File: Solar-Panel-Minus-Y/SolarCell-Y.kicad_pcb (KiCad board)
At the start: 6 copper layers, 64 x 58 mm, 67 parts, among them IC2 TSL2561, J1 XF2M-1015-1A, J3 BATTERY CONNECTOR, J4 B2B-PH-SM4-TB_LF__SN_, U2 Value, U3 SW_SPDT, U4 SW_SPDT

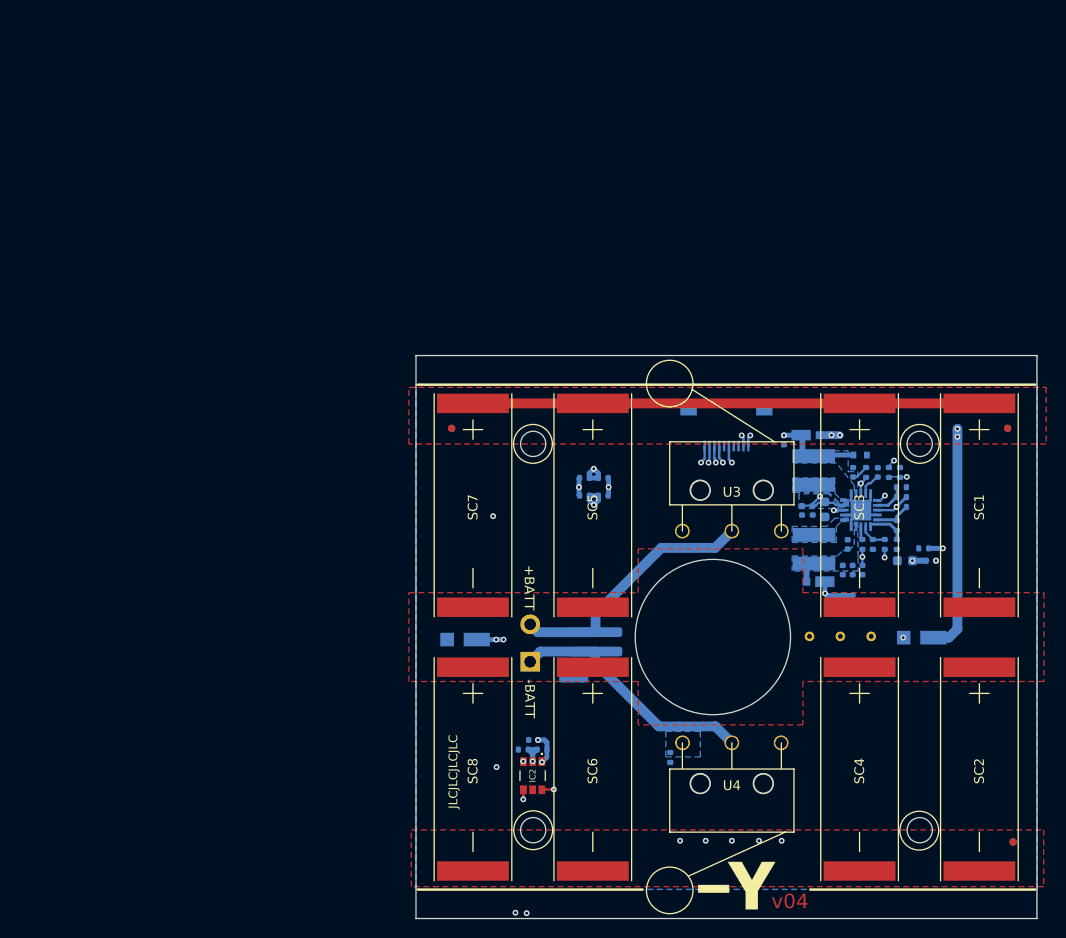
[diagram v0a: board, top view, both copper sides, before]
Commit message: Made Requested Changes
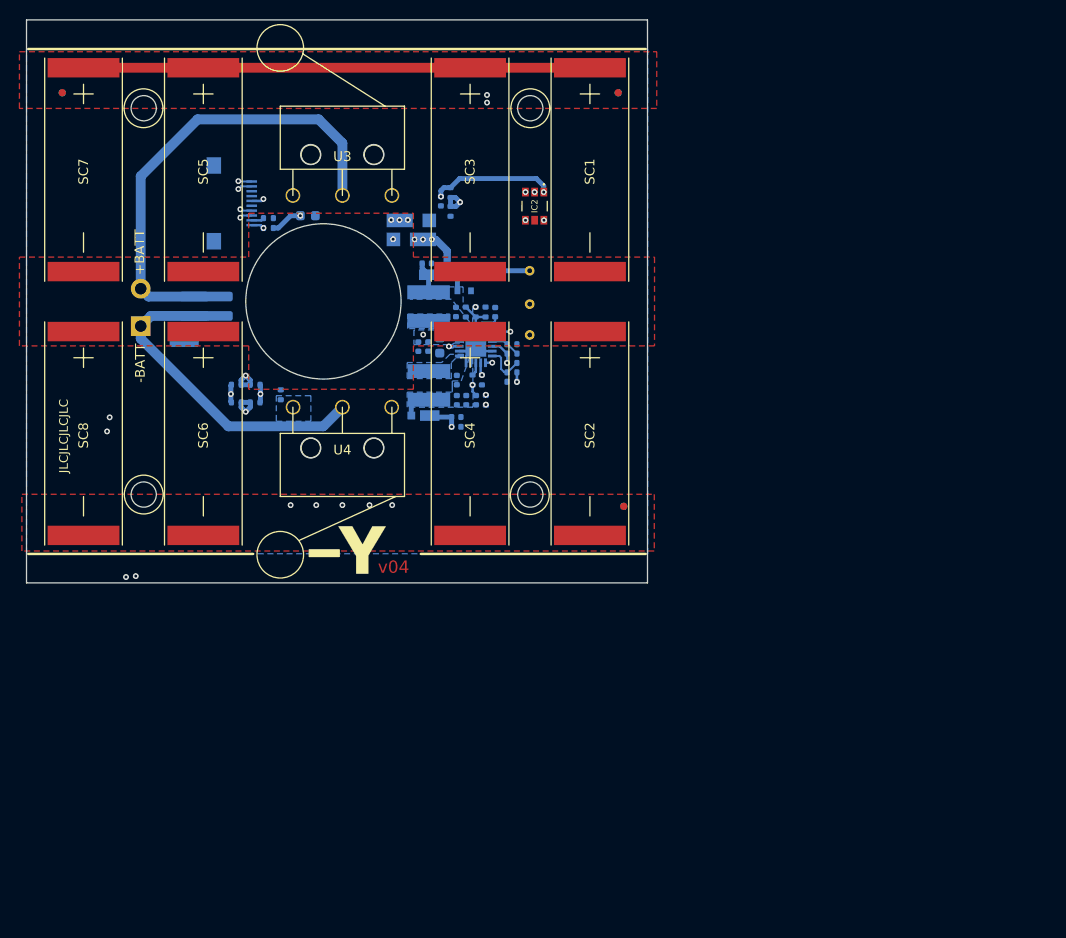
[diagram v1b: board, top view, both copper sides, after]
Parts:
- moved Ref** 77.4 mm to (97.4, 82.7), turned to 180 degrees
- moved R14 76.4 mm to (97.8, 56.9), turned to 0 degrees
- moved R15 75.6 mm to (97.8, 55.8), turned to 0 degrees
- moved C6 71.0 mm to (101.9, 55.6), turned to 0 degrees
- moved D11 66.7 mm to (112.5, 58.0)
- moved IC2 58.7 mm to (125.2, 54.6)
- moved R17 58.1 mm to (116.6, 53.2), turned to 90 degrees
- moved C5 56.3 mm to (115.6, 54.1), turned to 90 degrees
- moved R18 56.0 mm to (116.6, 55.1), turned to 90 degrees
- moved J1 54.9 mm to (96.1, 54.3), turned to 90 degrees
- moved R1000 54.8 mm to (99.1, 74.0), turned to 90 degrees
- moved REF** 53.0 mm to (134.4, 85.5) (x2)
- moved SC1 53.0 mm to (130.9, 40.4)
- moved SC2 53.0 mm to (130.9, 67.5)
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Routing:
- net BATT_P: track 40.5 -> 5.94 mm, vias 2 -> 1
- net BATT_N: track 31.5 -> 1.31 mm, vias 2 -> 0
- net SCL1: track 54.0 -> 31.4 mm
- net VSOLAR: track 34.7 -> 12.4 mm, vias 1 -> 0
- net Net-(J3-Pad2): track 26.5 -> 48.3 mm
- net /VBAT: track 12.7 -> 32.2 mm
- net SDA1: track 49.6 -> 33.9 mm
- net Net-(IC2-Pad2): track 2.96 -> 11.6 mm, vias 1 -> 2
- net Net-(C10-Pad1): track 15.8 -> 7.45 mm
- net Net-(J3-Pad1): track 25.8 -> 33.8 mm
- net COIL_P: track 23.6 -> 31.5 mm
- net Net-(R11-Pad1): track 8.95 -> 3.78 mm, vias 2 -> 0
- net COIL_N: track 21.9 -> 26.8 mm
- net Net-(D11-Pad2): track 5.25 -> 2.48 mm, vias 3 -> 4
- net /VSOLAR_FULL: track 77.7 -> 79.9 mm, vias 4 -> 5
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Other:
- rule pad_to_mask_clearance: 0.049 -> 0.0508
